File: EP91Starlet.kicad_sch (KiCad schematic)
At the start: 4 parts, among them M1 Module-mega-mcu64-0.1, M2 Module-wbo-0.5, M3 Module-vr-max9924-0.1, M4 Module-knock-0.2

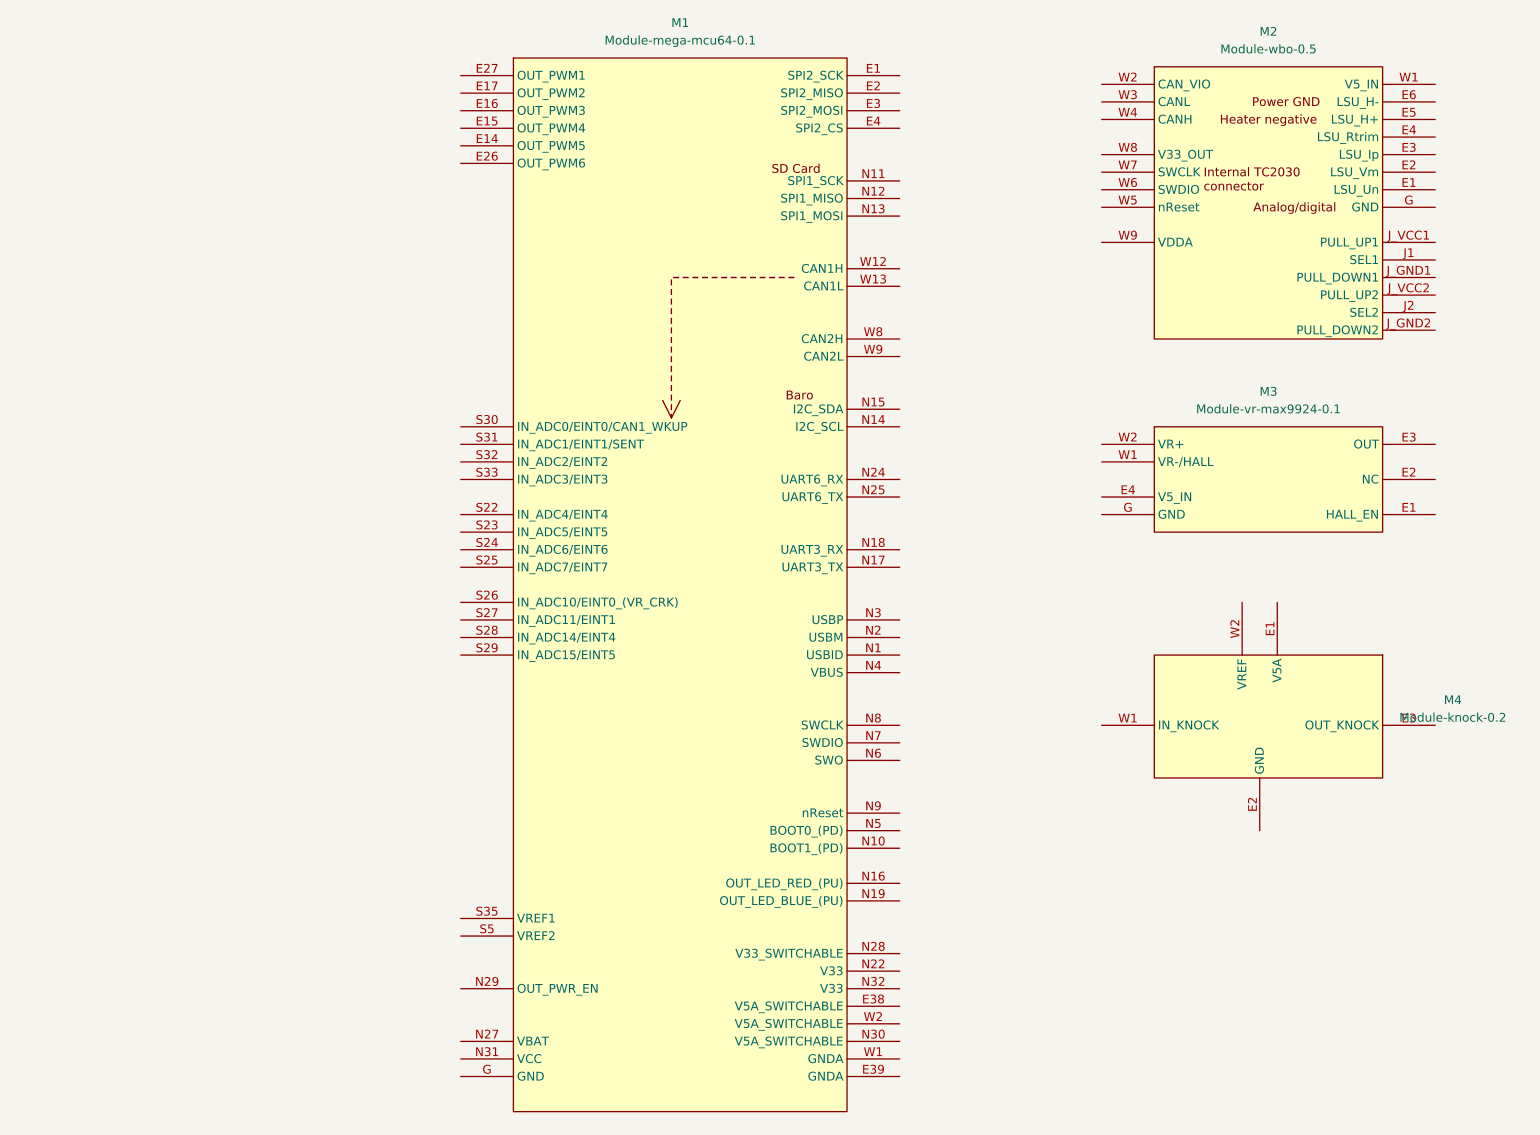
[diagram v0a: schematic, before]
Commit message: more testing
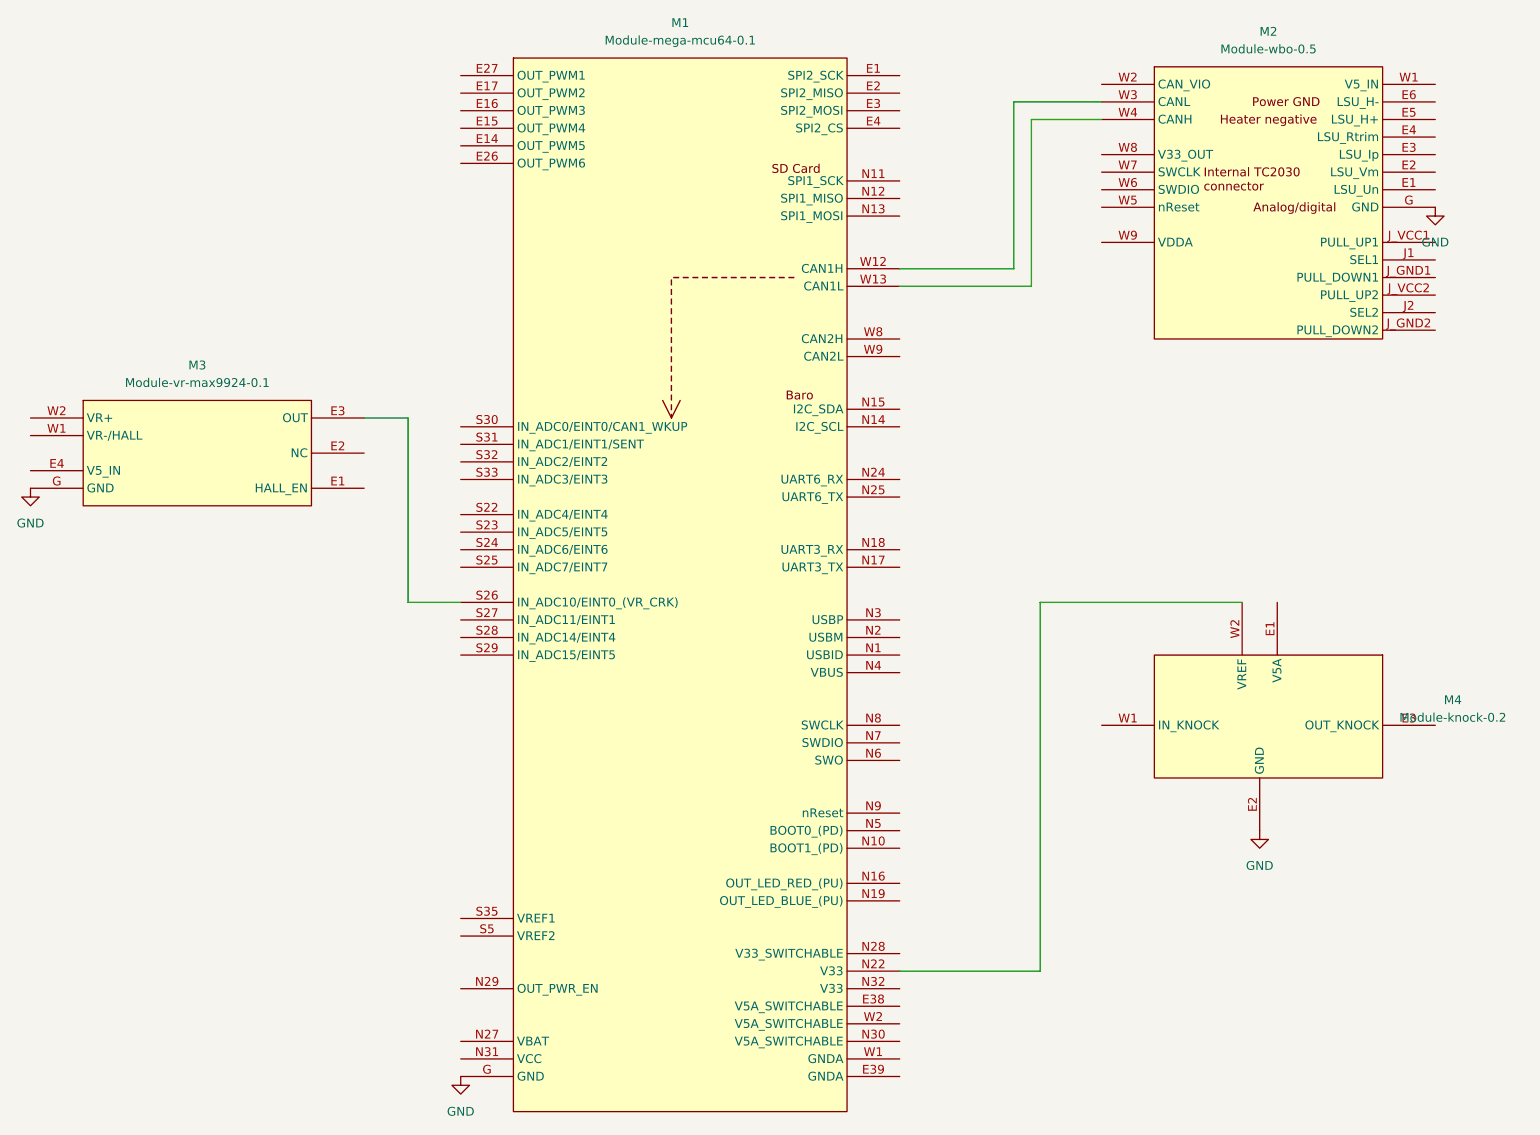
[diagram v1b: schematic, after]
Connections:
- net GND: now reaches M4.E2 (GND)
- net GND: now also M1.G (GND), M2.G (GND), M3.G (GND)
- net at M4.W2 (VREF): now also M1.N22 (V33)
- net at M1.S26 (IN_ADC10/EINT0_(VR_CRK)): now also M3.E3 (OUT)
- net at M1.W12 (CAN1H): now also M2.W3 (CANL)
- net at M1.W13 (CAN1L): now also M2.W4 (CANH)
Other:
- moved on the sheet: M3
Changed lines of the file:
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@@
 (kicad_sch (version 20230121) (generator eeschema)
   (paper "A4")
+  (wire (pts (xy 171.45 160.02) (xy 171.45 106.68))
+    (stroke (width 0) (type default))
+  )
+  (wire (pts (xy 167.64 34.29) (xy 167.64 58.42))
+    (stroke (width 0) (type default))
+  )
+  (wire (pts (xy 151.13 160.02) (xy 171.45 160.02))
+    (stroke (width 0) (type default))
+  )
+  (wire (pts (xy 180.34 34.29) (xy 167.64 34.29))
+    (stroke (width 0) (type default))
+  )
+  (wire (pts (xy 80.01 80.01) (xy 73.66 80.01))
+    (stroke (width 0) (type default))
+  )
+  (wire (pts (xy 87.63 106.68) (xy 80.01 106.68))
+    (stroke (width 0) (type default))
+  )
+  (wire (pts (xy 170.18 60.96) (xy 170.18 36.83))
+    (stroke (width 0) (type default))
+  )
+  (wire (pts (xy 167.64 58.42) (xy 151.13 58.42))
+    (stroke (width 0) (type default))
+  )
+  (wire (pts (xy 151.13 60.96) (xy 170.18 60.96))
+    (stroke (width 0) (type default))
+  )
+  (wire (pts (xy 80.01 106.68) (xy 80.01 80.01))
+    (stroke (width 0) (type default))
+  )
+  (wire (pts (xy 170.18 36.83) (xy 180.34 36.83))
+    (stroke (width 0) (type default))
+  )
+  (wire (pts (xy 171.45 106.68) (xy 200.66 106.68))
+    (stroke (width 0) (type default))
+  )
   (symbol (lib_id "knock:Module-knock-0.2") (at 187.96 114.3 0) (unit 1)
     (in_bom yes) (on_board yes) (dnp no) (fields_autoplaced)
@@
         (path "/10fbc709-889c-4565-8161-129ca9f0b73f"
           (reference "M4") (unit 1)
+        )
+      )
+    )
+  )
+  (symbol (lib_id "power:GND") (at 203.2 139.7 0) (unit 1)
+    (in_bom yes) (on_board yes) (dnp no) (fields_autoplaced)
+    (property "Reference" "#PWR03" (at 203.2 146.05 0)
+      (effects (font (size 1.27 1.27)) hide)
+    )
+    (property "Value" "GND" (at 203.2 144.78 0)
+      (effects (font (size 1.27 1.27)))
+    )
+    (property "Footprint" "" (at 203.2 139.7 0)
+      (effects (font (size 1.27 1.27)) hide)
+    )
+    (property "Datasheet" "" (at 203.2 139.7 0)
+      (effects (font (size 1.27 1.27)) hide)
+    )
+    (pin "1")
+    (instances
+      (project "EP91Starlet"
+        (path "/10fbc709-889c-4565-8161-129ca9f0b73f"
+          (reference "#PWR03") (unit 1)
+        )
+      )
+    )
+  )
+  (symbol (lib_id "power:GND") (at 228.6 49.53 0) (unit 1)
+    (in_bom yes) (on_board yes) (dnp no) (fields_autoplaced)
+    (property "Reference" "#PWR04" (at 228.6 55.88 0)
+      (effects (font (size 1.27 1.27)) hide)
+    )
+    (property "Value" "GND" (at 228.6 54.61 0)
+      (effects (font (size 1.27 1.27)))
+    )
+    (property "Footprint" "" (at 228.6 49.53 0)
+      (effects (font (size 1.27 1.27)) hide)
+    )
+    (property "Datasheet" "" (at 228.6 49.53 0)
+      (effects (font (size 1.27 1.27)) hide)
+    )
+    (pin "1")
+    (instances
+      (project "EP91Starlet"
+        (path "/10fbc709-889c-4565-8161-129ca9f0b73f"
+          (reference "#PWR04") (unit 1)
+        )
+      )
+    )
+  )
+  (symbol (lib_id "power:GND") (at 25.4 90.17 0) (unit 1)
+    (in_bom yes) (on_board yes) (dnp no) (fields_autoplaced)
+    (property "Reference" "#PWR01" (at 25.4 96.52 0)
+      (effects (font (size 1.27 1.27)) hide)
+    )
+    (property "Value" "GND" (at 25.4 95.25 0)
+      (effects (font (size 1.27 1.27)))
+    )
+    (property "Footprint" "" (at 25.4 90.17 0)
+      (effects (font (size 1.27 1.27)) hide)
+    )
+    (property "Datasheet" "" (at 25.4 90.17 0)
+      (effects (font (size 1.27 1.27)) hide)
+    )
+    (pin "1")
+    (instances
+      (project "EP91Starlet"
+        (path "/10fbc709-889c-4565-8161-129ca9f0b73f"
+          (reference "#PWR01") (unit 1)
+        )
+      )
+    )
+  )
+  (symbol (lib_id "power:GND") (at 87.63 175.26 0) (unit 1)
+    (in_bom yes) (on_board yes) (dnp no) (fields_autoplaced)
+    (property "Reference" "#PWR02" (at 87.63 181.61 0)
+      (effects (font (size 1.27 1.27)) hide)
+    )
+    (property "Value" "GND" (at 87.63 180.34 0)
+      (effects (font (size 1.27 1.27)))
+    )
+    (property "Footprint" "" (at 87.63 175.26 0)
+      (effects (font (size 1.27 1.27)) hide)
+    )
+    (property "Datasheet" "" (at 87.63 175.26 0)
+      (effects (font (size 1.27 1.27)) hide)
+    )
+    (pin "1")
+    (instances
+      (project "EP91Starlet"
+        (path "/10fbc709-889c-4565-8161-129ca9f0b73f"
+          (reference "#PWR02") (unit 1)
         )
       )
@@
     )
   )
-  (symbol (lib_id "vr-max9924:Module-vr-max9924-0.1") (at 187.96 81.28 0) (unit 1)
-    (in_bom yes) (on_board yes) (dnp no) (fields_autoplaced)
-    (property "Reference" "M3" (at 204.47 76.2 0)
-      (effects (font (size 1.27 1.27)))
-    )
-    (property "Value" "Module-vr-max9924-0.1" (at 204.47 78.74 0)
-      (effects (font (size 1.27 1.27)))
-    )
-    (property "Footprint" "0.3:vr-max9924" (at 213.36 80.01 0)
-      (effects (font (size 1.27 1.27)) hide)
-    )
-    (property "Datasheet" "" (at 187.96 81.28 0)
-      (effects (font (size 1.27 1.27)) hide)
-    )
+  (symbol (lib_id "vr-max9924:Module-vr-max9924-0.1") (at 33.02 77.47 0) (unit 1)
+    (in_bom yes) (on_board yes) (dnp no) (fields_autoplaced)
+    (property "Reference" "M3" (at 49.53 72.39 0)
+      (effects (font (size 1.27 1.27)))
+    )
+    (property "Value" "Module-vr-max9924-0.1" (at 49.53 74.93 0)
+      (effects (font (size 1.27 1.27)))
+    )
+    (property "Footprint" "0.3:vr-max9924" (at 58.42 76.2 0)
+      (effects (font (size 1.27 1.27)) hide)
+    )
+    (property "Datasheet" "" (at 33.02 77.47 0)
+      (effects (font (size 1.27 1.27)) hide)
+    )
